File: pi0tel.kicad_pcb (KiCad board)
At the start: 2 copper layers, 65 x 30 mm, 14 parts, among them J1 DIN-5_180degree, J2 RPi_GPIO, Q1 BSS138, U1 LM2596S-5

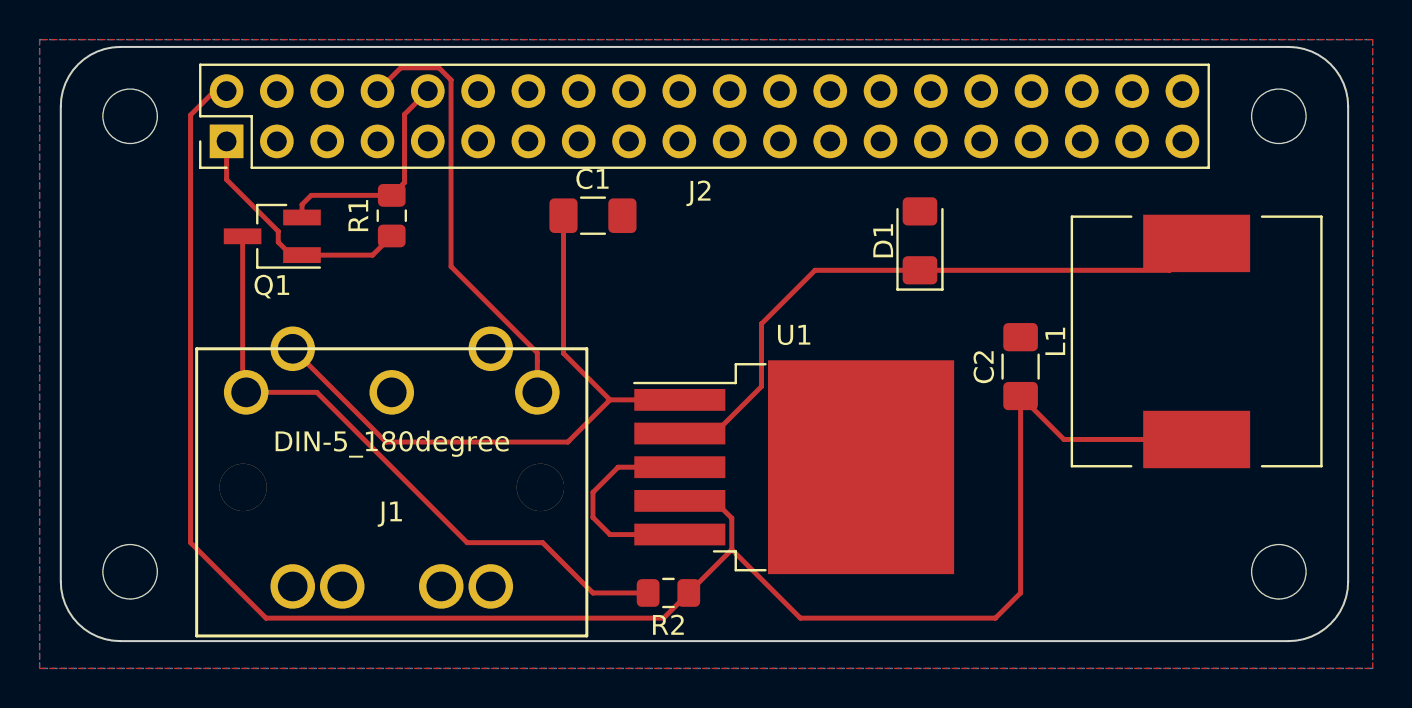
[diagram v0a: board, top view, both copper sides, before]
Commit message: getting there
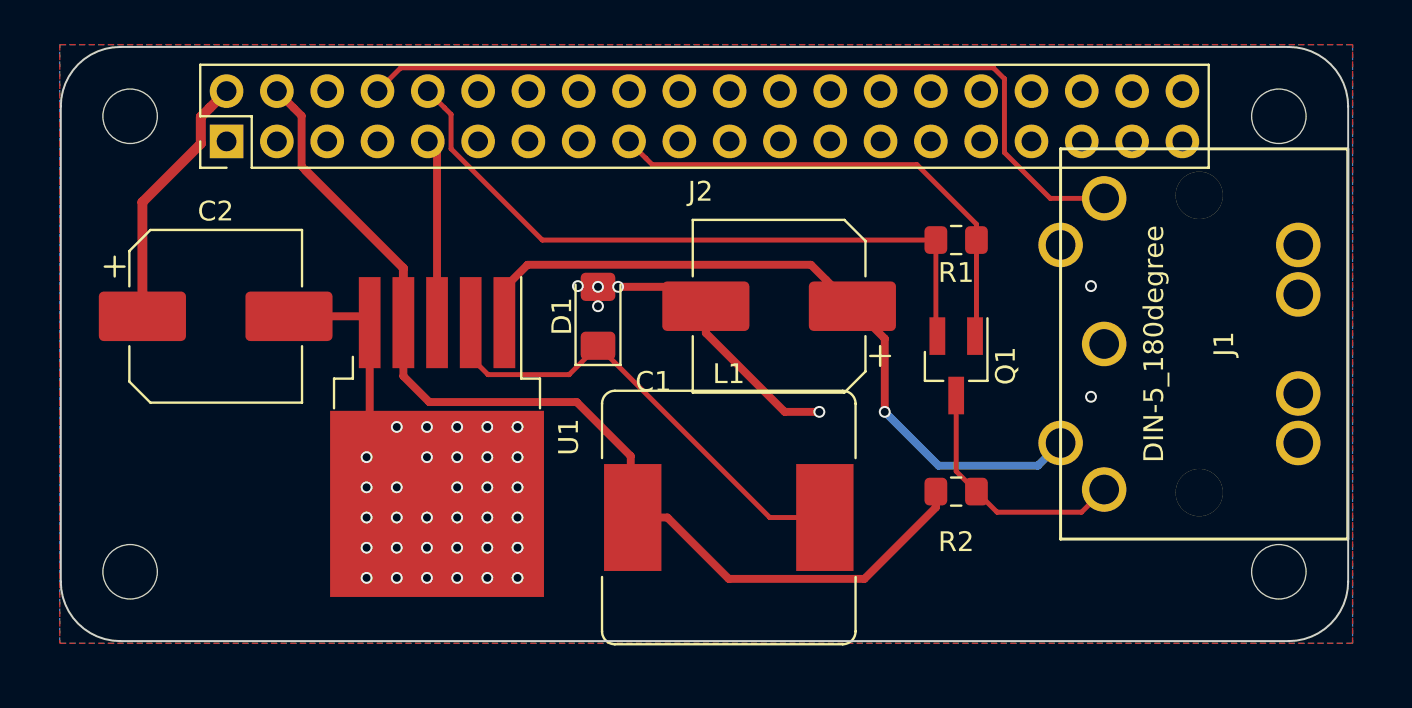
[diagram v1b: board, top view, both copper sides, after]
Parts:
- C1: value 680uF -> 270uF; footprint Capacitor_SMD:C_1206_3216Metric_Pad1.42x1.75mm_HandSolder -> Capacitor_SMD:CP_Elec_8x10.5
- C2: value 220uF -> 470uF; footprint Capacitor_SMD:C_1206_3216Metric_Pad1.42x1.75mm_HandSolder -> Capacitor_SMD:CP_Elec_8x10.5
- L1: value 33uH -> 68uH; footprint Inductor_SMD:L_12x12mm_H6mm -> Inductor_SMD:L_Bourns_SRR1260
- moved J1 41.7 mm to (70.2, 39.5), turned to 270 degrees
- moved C2 40.7 mm to (20.3, 38.1), turned to 0 degrees
- moved Q1 35.1 mm to (57.7, 40.6), turned to 270 degrees
- moved R1 28.5 mm to (57.7, 34.3), turned to 180 degrees
- moved L1 25.2 mm to (46.2, 48.3), turned to 0 degrees
- moved U1 18.1 mm to (31.5, 44.2), turned to 270 degrees
- moved D1 16.7 mm to (39.6, 38.1)
- moved R2 15.4 mm to (57.7, 47.0), turned to 0 degrees
- moved C1 10.5 mm to (48.8, 37.6), turned to 180 degrees
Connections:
- J2 pad 1: +3V3 -> Net-(J2-Pad1)
- J2 pad 17: Net-(J2-Pad17) -> +3V3
- J2 pad 25: GND -> Net-(J2-Pad25)
- J2 pad 4: Net-(J2-Pad4) -> +5V
- J2 pad 9: Net-(J2-Pad9) -> GND
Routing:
- net +5V: track 95.1 -> 65.4 mm
- net GND: track 10.9 -> 38.7 mm, vias 0 -> 40
- net /PiRx: track 11.4 -> 34.7 mm
- net /MinitelTx: track 32.7 -> 12.6 mm
- net /MinitelRx: track 22.0 -> 42.1 mm
- net +3V3: track 12.6 -> 25.0 mm
- net Net-(D1-Pad1): track 31.9 -> 25.7 mm
- net /MinitelVcc: track 32.7 -> 37.2 mm, vias 0 -> 1
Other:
- net class Largish added: clearance 0.2, trace_width 0.4, via_dia 0.6, via_drill 0.4
